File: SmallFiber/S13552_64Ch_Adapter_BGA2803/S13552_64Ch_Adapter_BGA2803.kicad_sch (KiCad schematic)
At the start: 11 parts, among them J1 ERM6-30-01.5-L-DV-A-K-TR, J2 ERM6-30-01.5-L-DV-A-K-TR

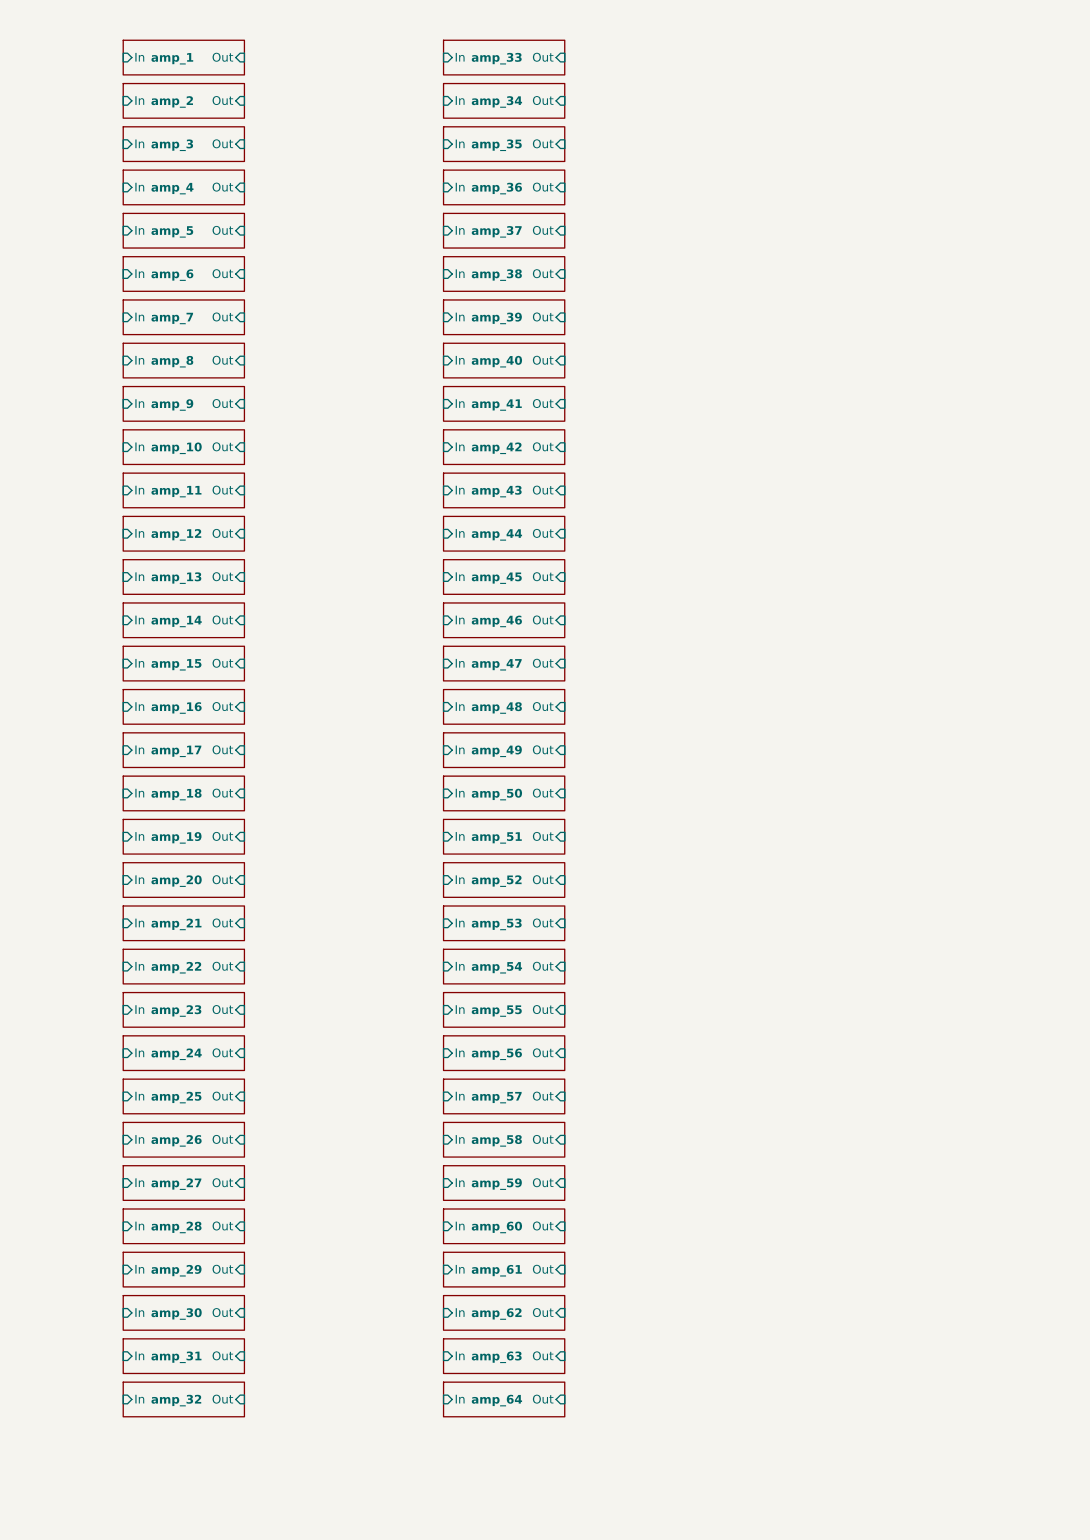
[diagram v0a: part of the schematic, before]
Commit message: .
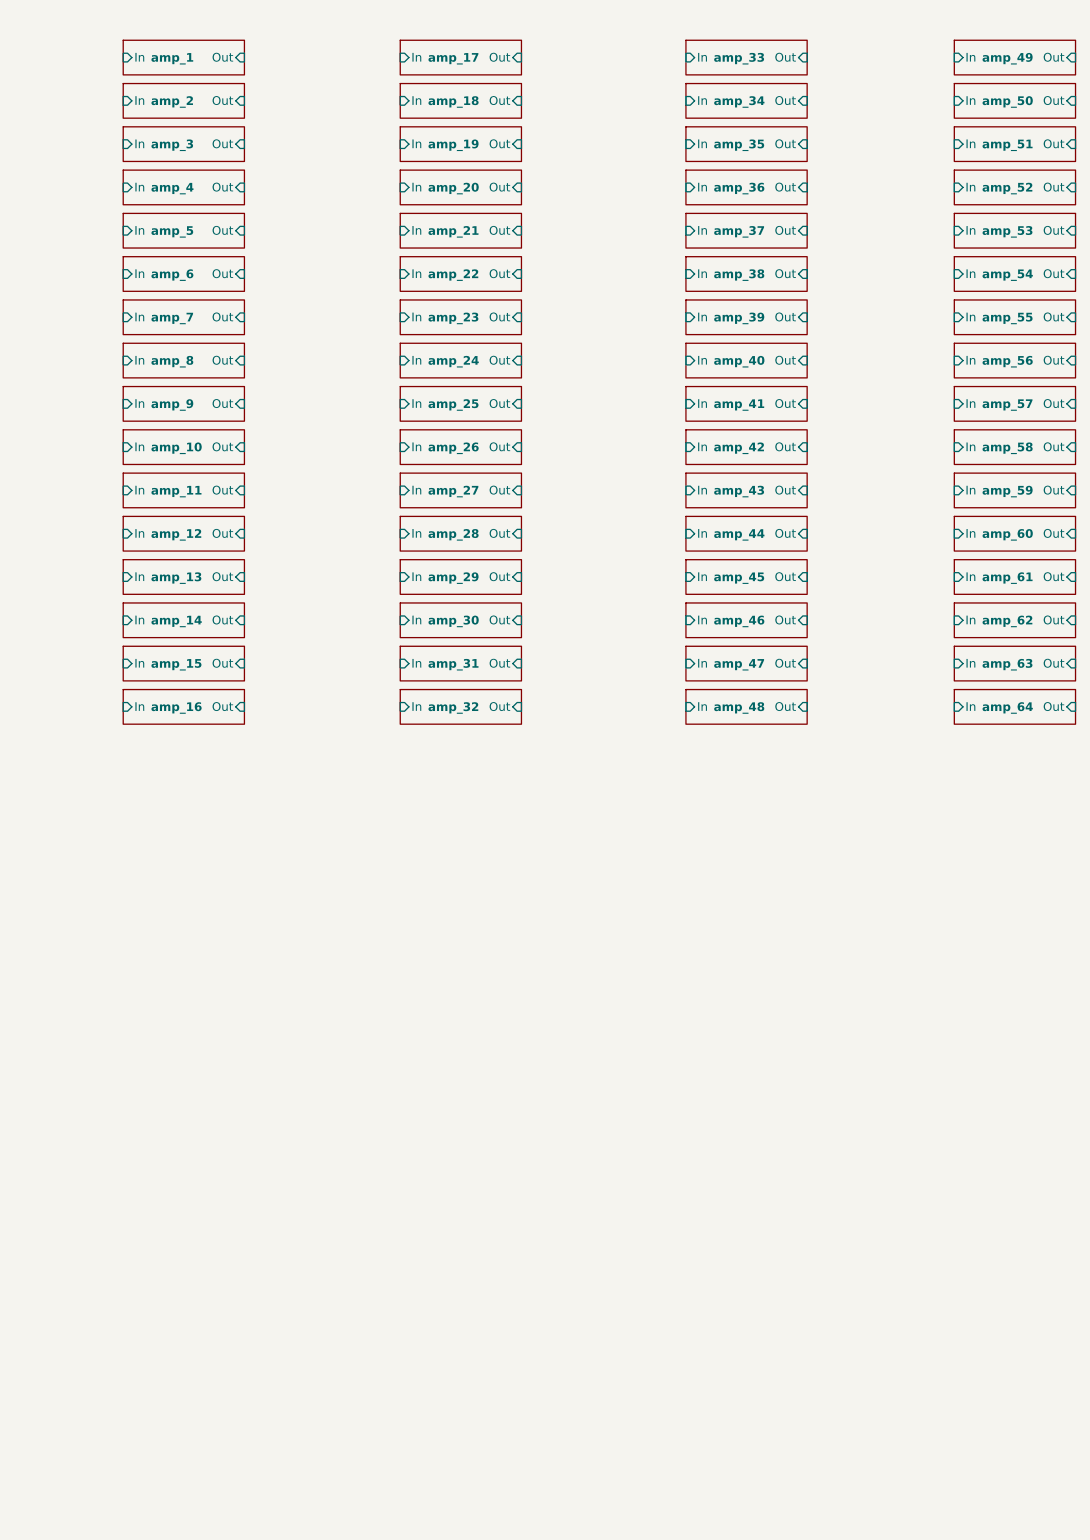
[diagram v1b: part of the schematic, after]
